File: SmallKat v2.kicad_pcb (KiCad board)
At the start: 2 copper layers, 90 x 56 mm, 64 parts, among them IC1 TPS562201DDCR, J1 Conn_01x06_Male, J10 Conn_01x03_Male, J11 Conn_01x03_Male, J12 Conn_01x03_Male, J13 Conn_01x03_Male, J14 Conn_01x03_Male, J15 Conn_01x03_Male, J16 Conn_01x03_Male, J17 Conn_01x03_Male, J18 Conn_01x03_Male, J19 Conn_01x03_Male, J2 Conn_01x06_Male, J20 Conn_01x03_Male, J21 Conn_01x02_Male, J22 Conn_01x02_Male, J23 Conn_01x02_Male, J24 Conn_01x02_Male, J25 Conn_01x02_Male, J26 Conn_01x02_Male, J27 Conn_01x02_Male, J28 Conn_01x02_Male, J29 Conn_01x02_Male, J3 Conn_01x06_Male, J30 Conn_01x15_Female, J31 Conn_01x15_Female, J4 Conn_01x06_Male, J5 Conn_01x03_Male, J6 Conn_01x03_Male, J7 Conn_01x03_Male, J8 Conn_01x03_Male, J9 Conn_01x03_Male, U3 PCA9685BS, U4 BNO055, Y1 32.768kHz

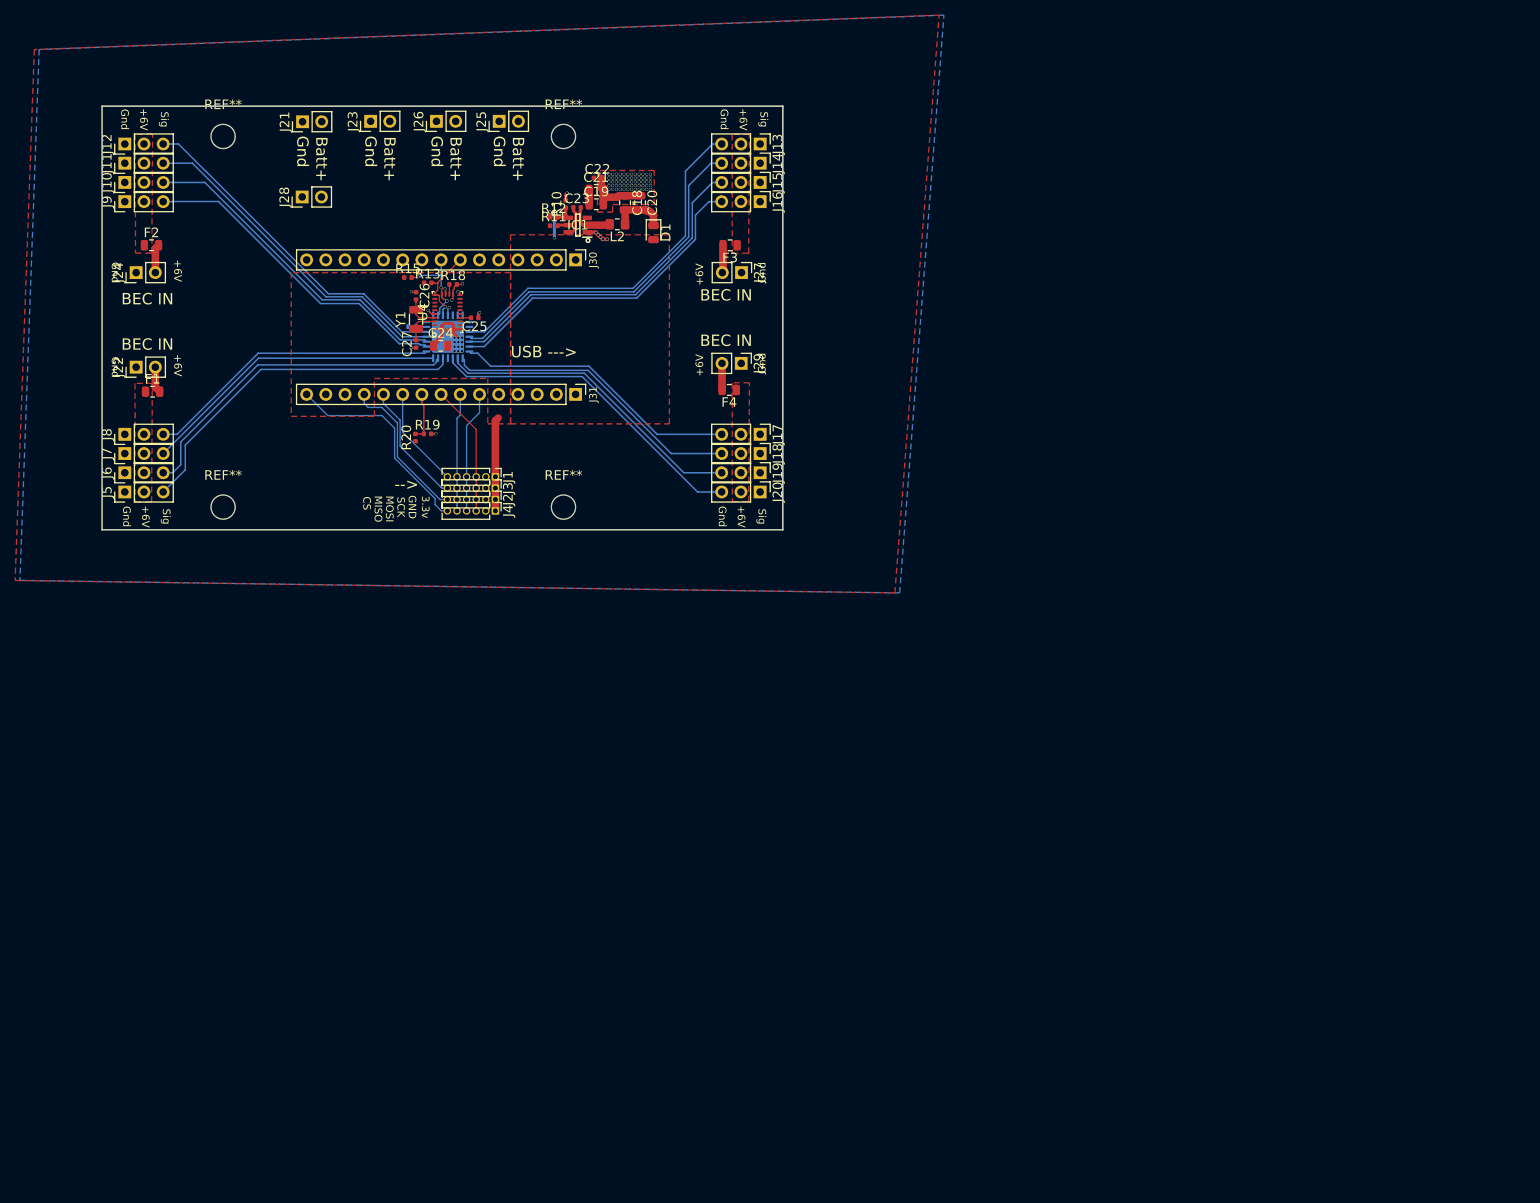
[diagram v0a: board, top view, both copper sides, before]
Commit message: init
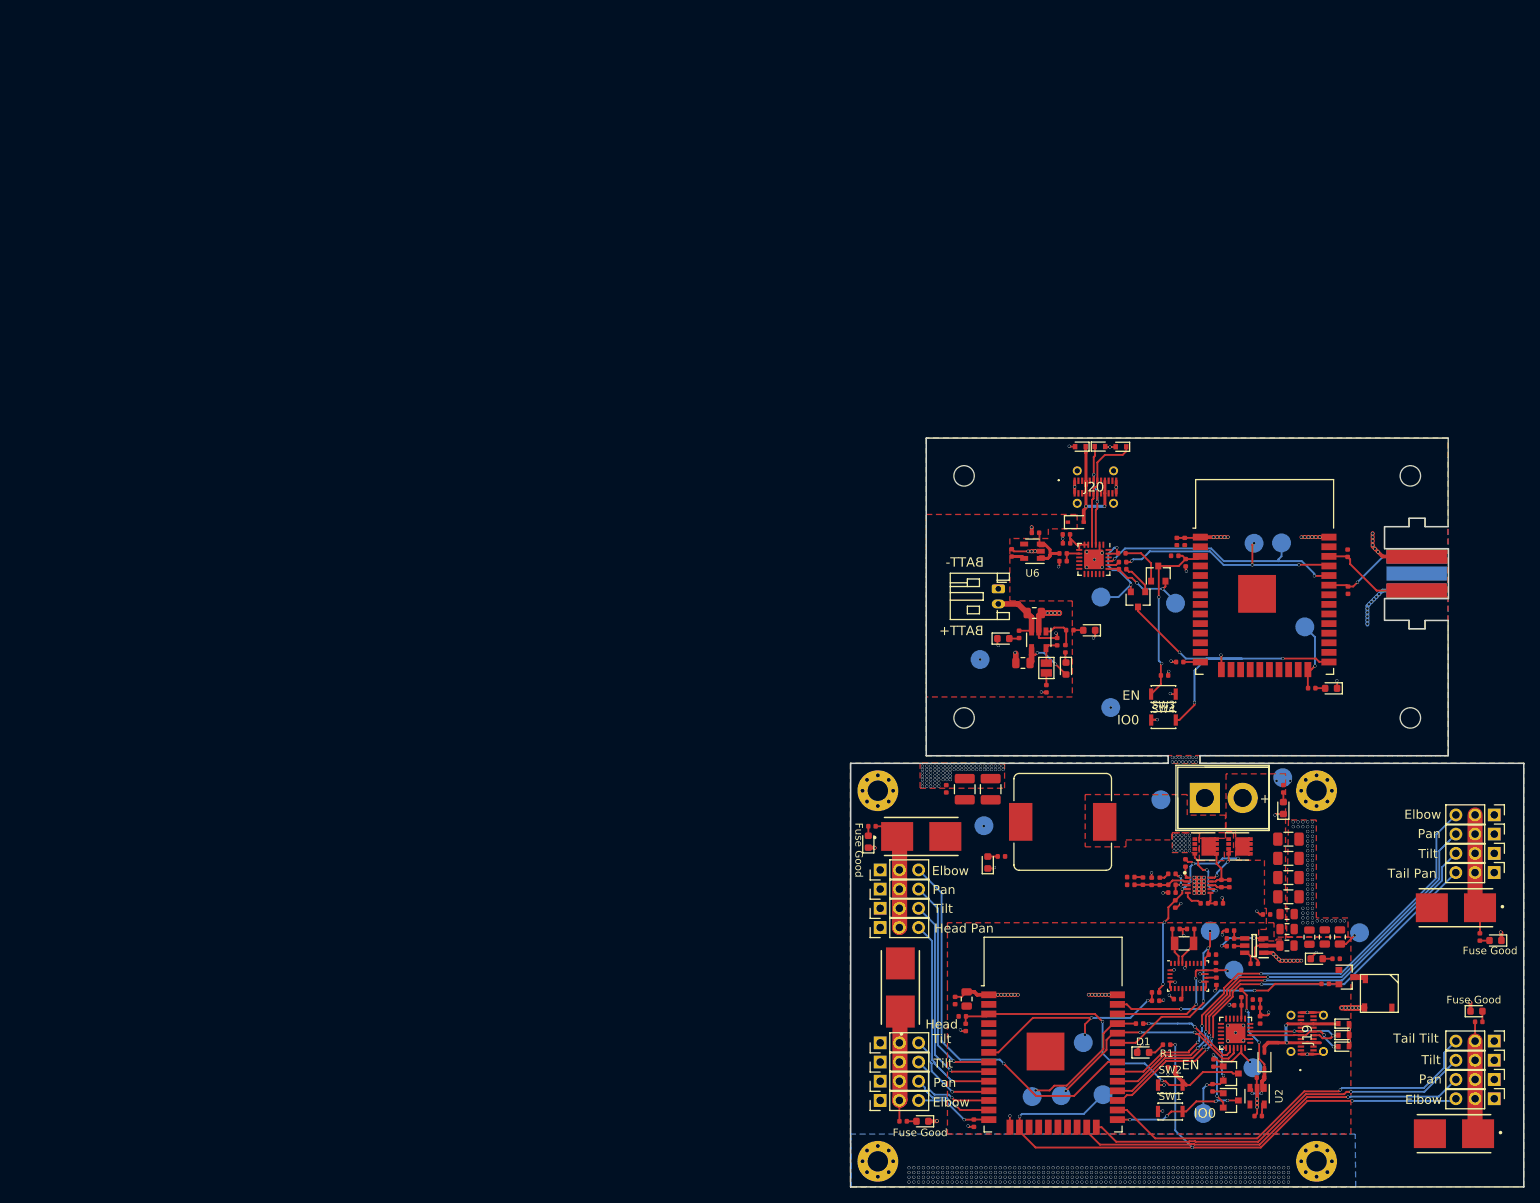
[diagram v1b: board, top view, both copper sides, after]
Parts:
- removed J21, J22, J23, J24, J25, J26, J27, J28, J29: Conn_01x02_Male, Connector_PinHeader_2.54mm:PinHeader_1x02_P2.54mm_Vertical
- removed J30, J31: Conn_01x15_Female, Connector_PinHeader_2.54mm:PinHeader_1x15_P2.54mm_Vertical
- removed REF** (x4): MountingHole_3.2mm_M3, MountingHole:MountingHole_3.2mm_M3
- added BZ1: Buzzer, KLJ-5030:KLJ-5030, F.Cu at (168.9, 117.3)
- added C1: 10uF, Capacitor_SMD:C_0805_2012Metric, F.Cu at (156.7, 108.8)
- added C10: 1000pF, Capacitor_SMD:C_0402_1005Metric, F.Cu at (136.0, 101.9)
- added C11: 100pF, Capacitor_SMD:C_0402_1005Metric, F.Cu at (141.4, 102.9)
- added C12: 10nF, Capacitor_SMD:C_0402_1005Metric, F.Cu at (141.4, 101.5)
- added C13: 1uF, Capacitor_SMD:C_0402_1005Metric, F.Cu at (141.9, 105.5)
- added C14: 4.7uF, Capacitor_SMD:C_0402_1005Metric, F.Cu at (147.7, 105.4)
- added C15: 470nF, Capacitor_SMD:C_0402_1005Metric, F.Cu at (148.0, 102.8)
- added C16: 10uF, Capacitor_SMD:C_1206_3216Metric, F.Cu at (156.8, 104.5)
- added C17: 47uF, Capacitor_SMD:C_1206_3216Metric, F.Cu at (156.8, 96.9)
- added C2: 10uF, Capacitor_SMD:C_0805_2012Metric, F.Cu at (156.7, 106.8)
- added C28: 0.1uF, Capacitor_SMD:C_0402_1005Metric, F.Cu at (152.6, 118.1)
- added C29: 0.1uF, Capacitor_SMD:C_0402_1005Metric, F.Cu at (153.1, 120.8)
- added C3: 22uF, Capacitor_SMD:C_0805_2012Metric, F.Cu at (161.6, 109.8)
- added C31: 0.1uF, Capacitor_SMD:C_0402_1005Metric, F.Cu at (141.4, 127.1)
- added C32: 0.1uF, Capacitor_SMD:C_0402_1005Metric, F.Cu at (114.2, 121.8)
- added C33: 10uF, Capacitor_SMD:C_0805_2012Metric, F.Cu at (121.7, 73.6)
- added C34: 10uF, Capacitor_SMD:C_0805_2012Metric, F.Cu at (123.2, 67.0)
- added C35: 1uF, Capacitor_SMD:C_0402_1005Metric, F.Cu at (123.4, 56.4)
- added C36: 22uF, Capacitor_SMD:C_0805_2012Metric, F.Cu at (163.7, 109.8)
- added C37: 1uF, Capacitor_SMD:C_0402_1005Metric, F.Cu at (120.2, 59.0)
- added C38: 0.1uF, Capacitor_SMD:C_0402_1005Metric, F.Cu at (143.1, 57.6)
- added C39: 4.7uF, Capacitor_SMD:C_0402_1005Metric, F.Cu at (142.1, 57.6)
- added C4: 0.1uF, Capacitor_SMD:C_0402_1005Metric, F.Cu at (153.9, 106.9)
- added C40: 0.1uF, Capacitor_SMD:C_0402_1005Metric, F.Cu at (127.5, 57.8)
- added C41: 0.1uF, Capacitor_SMD:C_0402_1005Metric, F.Cu at (127.5, 56.6)
- added C43: 0.1uF, Capacitor_SMD:C_0402_1005Metric, F.Cu at (140.5, 75.3)
- added C44: 0.1uF, Capacitor_SMD:C_0402_1005Metric, F.Cu at (143.3, 60.4)
- added C5: 22uF, Capacitor_SMD:C_0805_2012Metric, F.Cu at (159.6, 109.9)
- added C6: 0.1uF, Capacitor_SMD:C_0402_1005Metric, F.Cu at (152.3, 113.4)
- added C7: 0.1uF, Capacitor_SMD:C_0402_1005Metric, F.Cu at (142.2, 118.0)
- added C8: 10pF, Capacitor_SMD:C_0402_1005Metric, F.Cu at (143.9, 108.8)
- added C9: 10pF, Capacitor_SMD:C_0402_1005Metric, F.Cu at (142.0, 108.8)
- added D10: LED, LED_SMD:LED_0603_1608Metric, F.Cu at (119.2, 70.4)
- added D11: LED, LED_SMD:LED_0603_1608Metric, F.Cu at (127.4, 74.3)
- added D12: LED, LED_SMD:LED_0603_1608Metric, F.Cu at (130.5, 69.3)
- added D13: D_TVS, Diode_SMD:D_SOD-523, F.Cu at (129.3, 45.0)
- added D14: D_Schottky, Diode_SMD:D_SOD-323, F.Cu at (128.7, 55.0)
- added D15: D_TVS, Diode_SMD:D_SOD-523, F.Cu at (134.7, 45.0)
- added D16: D_TVS, Diode_SMD:D_SOD-523, F.Cu at (131.9, 45.0)
- added D17: LED, LED_SMD:LED_0603_1608Metric, F.Cu at (108.5, 134.2)
- added D18: LED, LED_SMD:LED_0603_1608Metric, F.Cu at (101.3, 97.2)
- added D19: LED, LED_SMD:LED_0603_1608Metric, F.Cu at (181.7, 119.7)
- added D2: LED, LED_SMD:LED_0603_1608Metric, F.Cu at (156.2, 92.8)
- added D20: LED, LED_SMD:LED_0603_1608Metric, F.Cu at (184.2, 110.3)
- added D3: LED, LED_SMD:LED_0603_1608Metric, F.Cu at (160.6, 112.7)
- added D4: LED, LED_SMD:LED_0603_1608Metric, F.Cu at (117.1, 100.0)
- added D5: D_TVS, Diode_SMD:D_SOD-523, F.Cu at (164.1, 121.3)
- added D6: D_Schottky, Diode_SMD:D_SOD-323, F.Cu at (153.7, 126.1)
- added D7: D_TVS, Diode_SMD:D_SOD-523, F.Cu at (164.1, 122.8)
- added D8: D_TVS, Diode_SMD:D_SOD-523, F.Cu at (164.1, 124.3)
- added D9: LED, LED_SMD:LED_0603_1608Metric, F.Cu at (162.5, 77.0)
- added H1: MountingHole_Pad, MountingHole:MountingHole_2.7mm_M2.5_Pad_Via, F.Cu at (160.6, 139.5)
- added H2: MountingHole_Pad, MountingHole:MountingHole_2.7mm_M2.5_Pad_Via, F.Cu at (102.6, 139.5)
- added H3: MountingHole_Pad, MountingHole:MountingHole_2.7mm_M2.5_Pad_Via, F.Cu at (160.6, 90.5)
- added H4: MountingHole_Pad, MountingHole:MountingHole_2.7mm_M2.5_Pad_Via, F.Cu at (102.6, 90.5)
- added H5: MountingHole, MountingHole:MountingHole_2.7mm_M2.5, F.Cu at (114.0, 48.9)
- added H6: MountingHole, MountingHole:MountingHole_2.7mm_M2.5, F.Cu at (173.0, 48.9)
- added H7: MountingHole, MountingHole:MountingHole_2.7mm_M2.5, F.Cu at (114.0, 80.9)
- added H8: MountingHole, MountingHole:MountingHole_2.7mm_M2.5, F.Cu at (173.0, 80.9)
- added IC2: TPS40192DRCT, TPS40192DRCT:SON50P300X300X100-11N, F.Cu at (145.0, 103.0)
- added JP1: Jumper_NO_Small, Jumper:SolderJumper-2_P1.3mm_Open_Pad1.0x1.5mm, F.Cu at (124.8, 74.3)
- added L1: 4.7uH, Inductor_SMD:L_0805_2012Metric, F.Cu at (156.6, 111.0)
- added Q1: BUK9M120-100EX, Package_SON:VSON-8_3.3x3.3mm_P0.65mm_NexFET, F.Cu at (150.4, 97.9)
- added Q2: BUK9M120-100EX, Package_SON:VSON-8_3.3x3.3mm_P0.65mm_NexFET, F.Cu at (145.9, 97.9)
- added Q3: MMBT3904, Package_TO_SOT_SMD:SOT-23, F.Cu at (149.2, 127.9)
- added Q4: MMBT3904, Package_TO_SOT_SMD:SOT-23, F.Cu at (149.2, 131.4)
- added Q5: MMBT3904, Package_TO_SOT_SMD:SOT-23, F.Cu at (139.6, 61.8)
- added Q6: MMBT3904, Package_TO_SOT_SMD:SOT-23, F.Cu at (137.0, 65.2)
- added Q7: 2N3905, Package_TO_SOT_SMD:SOT-23, F.Cu at (164.5, 115.1)
- added R1: R, Resistor_SMD:R_0402_1005Metric, F.Cu at (140.7, 124.1)
- added R16: 3.9k, Resistor_SMD:R_0402_1005Metric, F.Cu at (141.4, 104.0)
- added R17: 100k, Resistor_SMD:R_0402_1005Metric, F.Cu at (143.2, 100.1)
- added R2: 10K, Resistor_SMD:R_0402_1005Metric, F.Cu at (139.3, 118.3)
- added R21: 10K, Resistor_SMD:R_0402_1005Metric, F.Cu at (115.3, 134.5)
- added R22: 10K, Resistor_SMD:R_0402_1005Metric, F.Cu at (150.6, 117.3)
- added R23: 20K, Resistor_SMD:R_0402_1005Metric, F.Cu at (150.2, 118.9)
- added R24: 470R, Resistor_SMD:R_0402_1005Metric, F.Cu at (137.2, 121.3)
- added R25: 10K, Resistor_SMD:R_0402_1005Metric, F.Cu at (146.9, 126.5)
- added R26: 10K, Resistor_SMD:R_0402_1005Metric, F.Cu at (146.8, 129.8)
- added R27: 10K, Resistor_SMD:R_0402_1005Metric, F.Cu at (113.7, 120.3)
- added R28: 330R, Resistor_SMD:R_0402_1005Metric, F.Cu at (159.9, 76.9)
- added R29: 10K, Resistor_SMD:R_0402_1005Metric, F.Cu at (164.7, 59.1)
- added R3: 6.2k, Resistor_SMD:R_0402_1005Metric, F.Cu at (139.3, 117.2)
- added R30: 10K, Resistor_SMD:R_0402_1005Metric, F.Cu at (164.7, 64.0)
- added R31: 330R, Resistor_SMD:R_0402_1005Metric, F.Cu at (121.2, 69.8)
- added R32: 10K, Resistor_SMD:R_0402_1005Metric, F.Cu at (126.3, 70.8)
- added R33: 2.5K, Resistor_SMD:R_0402_1005Metric, F.Cu at (124.8, 77.0)
- added R34: 470R, Resistor_SMD:R_0402_1005Metric, F.Cu at (127.4, 71.7)
- added R35: 470R, Resistor_SMD:R_0402_1005Metric, F.Cu at (127.9, 69.3)
- added R36: 10K, Resistor_SMD:R_0402_1005Metric, F.Cu at (142.5, 73.5)
- added R37: 10K, Resistor_SMD:R_0402_1005Metric, F.Cu at (127.1, 59.1)
- added R38: 20K, Resistor_SMD:R_0402_1005Metric, F.Cu at (127.0, 60.1)
- added R39: 470R, Resistor_SMD:R_0402_1005Metric, F.Cu at (134.9, 60.3)
- added R4: 10K, Resistor_SMD:R_0402_1005Metric, F.Cu at (147.3, 113.7)
- added R40: 10K, Resistor_SMD:R_0402_1005Metric, F.Cu at (134.8, 59.1)
- added R41: 10K, Resistor_SMD:R_0402_1005Metric, F.Cu at (134.9, 61.2)
- added R42: 10K, Resistor_SMD:R_0402_1005Metric, F.Cu at (141.8, 59.4)
- added R43: 10K, Resistor_SMD:R_0402_1005Metric, F.Cu at (161.7, 116.0)
- added R44: R, Resistor_SMD:R_0402_1005Metric, F.Cu at (105.9, 134.2)
- added R45: R, Resistor_SMD:R_0402_1005Metric, F.Cu at (101.8, 95.2)
- added R46: R, Resistor_SMD:R_0402_1005Metric, F.Cu at (182.0, 121.0)
- added R47: R, Resistor_SMD:R_0402_1005Metric, F.Cu at (182.2, 109.8)
- added R5: 10K, Resistor_SMD:R_0402_1005Metric, F.Cu at (146.8, 112.2)
- added R6: 4.7K, Resistor_SMD:R_0402_1005Metric, F.Cu at (156.2, 90.2)
- added R7: 330R, Resistor_SMD:R_0402_1005Metric, F.Cu at (163.1, 112.7)
- added R8: 10K, Resistor_SMD:R_0402_1005Metric, F.Cu at (149.2, 109.0)
- added R9: 33.2K, Resistor_SMD:R_0402_1005Metric, F.Cu at (149.2, 110.0)
- added SW1: SW_SPST, Button_Switch_SMD:SW_SPST_CK_KXT3, F.Cu at (141.2, 132.9)
- added SW2: SW_SPST, Button_Switch_SMD:SW_SPST_CK_KXT3, F.Cu at (141.2, 129.4)
- added SW3: SW_SPST, Button_Switch_SMD:SW_SPST_CK_KXT3, F.Cu at (140.3, 81.2)
- added SW4: SW_SPST, Button_Switch_SMD:SW_SPST_CK_KXT3, F.Cu at (140.3, 77.7)
- added TP1: TestPoint, TestPoint:TestPoint_Pad_D2.5mm, B.Cu at (132.3, 130.7)
- added TP10: TestPoint, TestPoint:TestPoint_Pad_D2.5mm, B.Cu at (126.8, 130.8)
- added TP11: TestPoint, TestPoint:TestPoint_Pad_D2.5mm, B.Cu at (152.1, 127.1)
- added TP12: TestPoint, TestPoint:TestPoint_Pad_D2.5mm, B.Cu at (145.6, 133.2)
- added TP13: TestPoint, TestPoint:TestPoint_Pad_D2.5mm, B.Cu at (152.3, 57.8)
- added TP14: TestPoint, TestPoint:TestPoint_Pad_D2.5mm, B.Cu at (155.9, 57.7)
- added TP15: TestPoint, TestPoint:TestPoint_Pad_D2.5mm, B.Cu at (132.1, 64.9)
- added TP16: TestPoint, TestPoint:TestPoint_Pad_D2.5mm, B.Cu at (141.9, 65.7)
- added TP17: TestPoint, TestPoint:TestPoint_Pad_D2.5mm, B.Cu at (116.1, 73.2)
- added TP18: TestPoint, TestPoint:TestPoint_Pad_D2.5mm, B.Cu at (133.3, 79.5)
- added TP19: TestPoint, TestPoint:TestPoint_Pad_D2.5mm, B.Cu at (159.0, 68.8)
- added TP2: TestPoint, TestPoint:TestPoint_Pad_D2.5mm, B.Cu at (146.5, 109.0)
- added TP3: TestPoint, TestPoint:TestPoint_Pad_D2.5mm, B.Cu at (149.6, 114.2)
- added TP4: TestPoint, TestPoint:TestPoint_Pad_D2.5mm, B.Cu at (129.7, 123.8)
- added TP5: TestPoint, TestPoint:TestPoint_Pad_D2.5mm, B.Cu at (166.2, 109.3)
- added TP6: TestPoint, TestPoint:TestPoint_Pad_D2.5mm, B.Cu at (156.1, 88.8)
- added TP7: TestPoint, TestPoint:TestPoint_Pad_D2.5mm, B.Cu at (140.0, 91.7)
- added TP8: TestPoint, TestPoint:TestPoint_Pad_D2.5mm, B.Cu at (116.6, 95.1)
- added TP9: TestPoint, TestPoint:TestPoint_Pad_D2.5mm, B.Cu at (123.0, 130.9)
- added U1: BNO055, Package_LGA:LGA-28_5.2x3.8mm_P0.5mm, F.Cu at (143.6, 115.0)
- added U2: MIC5365-3.3YC5, Package_TO_SOT_SMD:SOT-23-5, F.Cu at (152.7, 130.9)
- added U5: MCP73831-2-OT, Package_TO_SOT_SMD:SOT-23-5, F.Cu at (123.8, 70.5)
- added U6: MIC5365-3.3YC5, Package_TO_SOT_SMD:SOT-23-5, F.Cu at (123.0, 58.8)
- added U7: ESP32-WROOM-32, RF_Module:ESP32-WROOM-32, F.Cu at (153.7, 65.2)
- added U8: CP2102N-A01-GQFN24, Package_DFN_QFN:QFN-24-1EP_4x4mm_P0.5mm_EP2.6x2.6mm, F.Cu at (131.1, 59.9)
- added U9: WIICHUCK, WIICHUCK:CHUCK, F.Cu at (169.5, 61.8)
- C18: value 22uF -> 10uF; footprint Capacitor_SMD:C_0805_2012Metric -> Capacitor_SMD:C_1206_3216Metric
- C19: value 10Uf -> 100uF; footprint Capacitor_SMD:C_0805_2012Metric -> Capacitor_SMD:C_1210_3225Metric
- C20: value 22uF -> 47uF; footprint Capacitor_SMD:C_0805_2012Metric -> Capacitor_SMD:C_1206_3216Metric
- C21: value 10uF -> 100uF; footprint Capacitor_SMD:C_0805_2012Metric -> Capacitor_SMD:C_1210_3225Metric
- C22, C23, C25: value 0.1uF -> 1uF
- C24: value 10uF -> 22uF
- C26: value 10pF -> 0.1uF
- C27: value 10pF -> 4.7uF
- D1: value DIODE -> LED; footprint Diode_SMD:D_0805_2012Metric -> LED_SMD:LED_0603_1608Metric
- F1, F2, F3, F4: footprint Fuse:Fuse_0805_2012Metric -> 01550900M:0154.250DR
- J1, J2, J3, J4: value Conn_01x06_Male -> Conn_01x03_Male; footprint Connector_PinHeader_1.27mm:PinHeader_1x06_P1.27mm_Vertical -> Connector_PinHeader_2.54mm:PinHeader_1x03_P2.54mm_Vertical
- J18: value Conn_01x03_Male -> Conn_01x02_Male; footprint Connector_PinHeader_2.54mm:PinHeader_1x03_P2.54mm_Vertical -> Connector_JST:JST_PH_S2B-PH-K_1x02_P2.00mm_Horizontal
- J19, J20: value Conn_01x03_Male -> USB_C_Receptacle; footprint Connector_PinHeader_2.54mm:PinHeader_1x03_P2.54mm_Vertical -> U263-241N-4BQC11-1:U263241N4BQC111
- J9: value Conn_01x03_Male -> Conn_01x02_Male; footprint Connector_PinHeader_2.54mm:PinHeader_1x03_P2.54mm_Vertical -> SmallKat ESP32:SHDR2W320P716_1X2_1574X813X1588P
- L2: value 4.7uH -> 1uH; footprint Inductor_SMD:L_0805_2012Metric_Pad1.15x1.40mm_HandSolder -> Inductor_SMD:L_Bourns_SRP1245A
- R12: value 61.63k -> 2.18k
- R13: value 10K -> 20k
- R14: value 10K -> 2.61k; moved to F.Cu
- R15: value 10K -> 4.22k
- R18, R19: value 10K -> 100k
- R20: value 6.2k -> 1K
- U3: value PCA9685BS -> ESP32-WROOM-32; footprint Package_DFN_QFN:QFN-28-1EP_6x6mm_P0.65mm_EP4.25x4.25mm -> RF_Module:ESP32-WROOM-32; moved to F.Cu
- U4: value BNO055 -> CP2102N-A01-GQFN24; footprint Package_LGA:LGA-28_5.2x3.8mm_P0.5mm -> Package_DFN_QFN:QFN-24-1EP_4x4mm_P0.5mm_EP2.6x2.6mm
- moved J10 217.8 mm to (184.1, 131.2), turned to 270 degrees
- moved J11 217.8 mm to (184.1, 128.7), turned to 270 degrees
- moved J12 217.8 mm to (184.1, 126.1), turned to 270 degrees
- moved J9 163.1 mm to (145.8, 91.5), turned to 0 degrees
- moved J13 153.2 mm to (184.1, 123.6)
- moved F3 151.5 mm to (178.7, 135.8)
- moved C25 147.9 mm to (152.8, 133.5)
- moved C23 146.3 mm to (153.1, 128.4), turned to 180 degrees
- moved C27 141.6 mm to (152.6, 119.2), turned to 0 degrees
- moved U4 141.2 mm to (149.9, 122.6), turned to 180 degrees
- moved J14 135.0 mm to (184.0, 101.3)
- moved R11 132.9 mm to (147.3, 115.7), turned to 270 degrees
- moved R10 131.7 mm to (149.2, 111.0), turned to 0 degrees
- moved J15 131.5 mm to (184.1, 98.8)
- moved Y1 130.8 mm to (143.0, 110.7), turned to 0 degrees
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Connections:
- C18 pad 1: GND -> +BATT
- C18 pad 2: Net-(C18-Pad2) -> GND
- C19 pad 1: +BATT -> +6V
- C20 pad 1: GND -> +BATT
- C20 pad 2: Net-(C18-Pad2) -> GND
- C21 pad 1: +BATT -> +6V
- C22 pad 1: +BATT -> +6V
- C23 pad 1: Net-(C23-Pad1) -> +5V
- C23 pad 2: Net-(C23-Pad2) -> GND
- C24 pad 1: GND -> +3V3
- C24 pad 2: +3V3 -> GND
- C25 pad 1: GND -> +3V3
- C25 pad 2: Net-(C25-Pad2) -> GND
- C26 pad 1: GND -> +3V3
- C26 pad 2: Net-(C26-Pad2) -> GND
- C27 pad 1: GND -> +3V3
- C27 pad 2: Net-(C27-Pad2) -> GND
- D1 pad 1: Net-(C18-Pad2) -> GND
- D1 pad 2: +5V -> Net-(D1-Pad2)
- F1 pad 1: +6V_1 -> Net-(F1-Pad1)
- F1 pad 2: +6V_IN1 -> +6V
- F2 pad 1: +6V_2 -> Net-(F2-Pad1)
- F2 pad 2: +6V_IN2 -> +6V
- F3 pad 1: +6V_3 -> Net-(F3-Pad1)
- F3 pad 2: +6V_IN3 -> +6V
- F4 pad 1: +6V_4 -> Net-(F4-Pad1)
- F4 pad 2: +6V_IN4 -> +6V
- IC1 pad 2: Net-(C23-Pad2) -> Net-(C6-Pad2)
- IC1 pad 6: Net-(C23-Pad1) -> Net-(C6-Pad1)
- J1 pad 1: +3V3 -> GND
- J1 pad 2: GND -> Net-(F1-Pad1)
- J1 pad 3: SCK -> /MainBoard/SERVO0
- J10 pad 2: +6V_2 -> Net-(F3-Pad1)
- J10 pad 3: SERVO5 -> /MainBoard/SERVO8
- J11 pad 2: +6V_2 -> Net-(F3-Pad1)
- J11 pad 3: SERVO6 -> /MainBoard/SERVO9
- J12 pad 2: +6V_2 -> Net-(F3-Pad1)
- J12 pad 3: SERVO7 -> /MainBoard/SERVO10
- J13 pad 2: +6V_3 -> Net-(F3-Pad1)
- J13 pad 3: SERVO8 -> /MainBoard/SERVO11
- J14 pad 2: +6V_3 -> Net-(F4-Pad1)
- J14 pad 3: SERVO9 -> /MainBoard/SERVO12
- J15 pad 2: +6V_3 -> Net-(F4-Pad1)
- J15 pad 3: SERVO10 -> /MainBoard/SERVO13
- J16 pad 2: +6V_3 -> Net-(F4-Pad1)
- J16 pad 3: SERVO11 -> /MainBoard/SERVO14
- J17 pad 2: +6V_4 -> Net-(F4-Pad1)
- J17 pad 3: SERVO12 -> /MainBoard/SERVO15
- J18 pad 2: +6V_4 -> +3V8
- J2 pad 1: +3V3 -> GND
- J2 pad 2: GND -> Net-(F1-Pad1)
- J2 pad 3: SCK -> /MainBoard/SERVO1
- J3 pad 1: +3V3 -> GND
- J3 pad 2: GND -> Net-(F1-Pad1)
- J3 pad 3: SCK -> /MainBoard/SERVO2
- J4 pad 1: +3V3 -> GND
- J4 pad 2: GND -> Net-(F1-Pad1)
- J4 pad 3: SCK -> /MainBoard/SERVO3
- J5 pad 2: +6V_1 -> Net-(F2-Pad1)
- J5 pad 3: SERVO0 -> /MainBoard/SERVO4
- J6 pad 2: +6V_1 -> Net-(F2-Pad1)
- J6 pad 3: SERVO1 -> /MainBoard/SERVO5
- J7 pad 2: +6V_1 -> Net-(F2-Pad1)
- J7 pad 3: SERVO2 -> /MainBoard/SERVO6
- J8 pad 2: +6V_1 -> Net-(F2-Pad1)
- J8 pad 3: SERVO3 -> /MainBoard/SERVO7
- J9 pad 2: +6V_2 -> +BATT
- L2 pad 1: Net-(C18-Pad2) -> Net-(C15-Pad1)
- L2 pad 2: Net-(C23-Pad2) -> +6V
- R10 pad 1: Net-(IC1-Pad4) -> +BATT
- R10 pad 2: GND -> Net-(IC1-Pad5)
- R11 pad 1: +BATT -> Net-(R11-Pad1)
- R11 pad 2: Net-(IC1-Pad5) -> GND
- R12 pad 1: +5V -> Net-(C11-Pad2)
- R12 pad 2: Net-(IC1-Pad4) -> GND
- R13 pad 1: +3V3 -> +6V
- R13 pad 2: SDA -> Net-(C11-Pad2)
- R14 pad 1: Net-(R14-Pad1) -> Net-(C11-Pad2)
- R14 pad 2: GND -> Net-(C10-Pad2)
- R15 pad 1: +3V3 -> Net-(C12-Pad2)
- R15 pad 2: SCL -> Net-(C11-Pad2)
- R18 pad 1: Net-(R18-Pad1) -> Net-(C14-Pad1)
- R18 pad 2: GND -> Net-(IC2-Pad5)
- R19 pad 1: BATTMONITOR -> Net-(C15-Pad1)
- R19 pad 2: GND -> Net-(C15-Pad2)
- R20 pad 1: +BATT -> +6V
- R20 pad 2: BATTMONITOR -> Net-(D4-Pad2)
- U3 pad 1: (no net) -> GND
- U3 pad 10: SERVO15 -> /MainBoard/SERVO4
- U3 pad 11: GND -> /MainBoard/SERVO3
- U3 pad 12: SERVO0 -> /MainBoard/SERVO2
- U3 pad 13: SERVO1 -> /MainBoard/SERVO1
- U3 pad 14: SERVO2 -> /MainBoard/SERVO0
- U3 pad 15: SERVO3 -> GND
- U3 pad 16: SERVO4 -> /MainBoard/SERVO8
- U3 pad 17: SERVO5 -> (no net)
- U3 pad 18: SERVO6 -> (no net)
- U3 pad 19: SERVO7 -> (no net)
- U3 pad 2: (no net) -> +3V3
- U3 pad 20: Net-(R14-Pad1) -> (no net)
- U3 pad 22: GND -> (no net)
- U3 pad 23: SCL -> /MainBoard/SERVO9
- U3 pad 24: SDA -> /MainBoard/SERVO10
- U3 pad 25: +3V3 -> /MainBoard/ESP32Module/IO0
- U3 pad 26: (no net) -> /MainBoard/SERVO11
- U3 pad 27: (no net) -> /MainBoard/SERVO12
- U3 pad 28: (no net) -> /MainBoard/SERVO13
- U3 pad 29: GND -> /MainBoard/SERVO14
- U3 pad 3: SERVO8 -> /MainBoard/ESP32Module/EN
- U3 pad 4: SERVO9 -> (no net)
- U3 pad 5: SERVO10 -> (no net)
- U3 pad 6: SERVO11 -> (no net)
- U3 pad 7: SERVO12 -> /MainBoard/BATTMONITOR
- U3 pad 8: SERVO13 -> /MainBoard/SERVO6
- U3 pad 9: SERVO14 -> /MainBoard/SERVO5
- U4 pad 15: GND -> (no net)
- U4 pad 16: GND -> (no net)
- U4 pad 17: Net-(R18-Pad1) -> (no net)
- U4 pad 18: GND -> (no net)
- U4 pad 19: SCL -> /MainBoard/ESP32Module/RTS
- U4 pad 20: SDA -> Net-(R24-Pad2)
- U4 pad 21: (no net) -> /MainBoard/ESP32Module/RXD
- U4 pad 23: (no net) -> /MainBoard/ESP32Module/DTR
- U4 pad 3: +3V3 -> /MainBoard/ESP32Module/USBD_P
- U4 pad 4: +3V3 -> /MainBoard/ESP32Module/USBD_N
- U4 pad 5: GND -> +3V3
- U4 pad 6: GND -> +3V3
- U4 pad 7: (no net) -> +3V3
- U4 pad 8: (no net) -> Net-(R22-Pad1)
- U4 pad 9: Net-(C25-Pad2) -> (no net)
- Y1 pad 1: Net-(C26-Pad2) -> Net-(C8-Pad2)
- Y1 pad 2: Net-(C27-Pad2) -> Net-(C9-Pad2)
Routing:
- net GND: track 28.5 -> 125.7 mm, vias 87 -> 315
- net /MainBoard/SERVO8: track 0.00 -> 90.6 mm, vias 0 -> 4
- net /MainBoard/SERVO15: track 0.00 -> 64.5 mm, vias 0 -> 3
- net /MainBoard/SERVO14: track 0.00 -> 62.8 mm, vias 0 -> 3
- net /MainBoard/SERVO13: track 0.00 -> 61.1 mm, vias 0 -> 3
- net /MainBoard/SERVO12: track 0.00 -> 59.7 mm, vias 0 -> 3
- net /MainBoard/SERVO9: track 0.00 -> 53.7 mm, vias 0 -> 1
- net /MainBoard/SERVO10: track 0.00 -> 52.8 mm, vias 0 -> 1
- net /MainBoard/SERVO11: track 0.00 -> 52.8 mm, vias 0 -> 1
- net /MainBoard/SERVO7: track 0.00 -> 52.0 mm, vias 0 -> 1
- net SERVO8: track 48.7 -> 0.00 mm
- net /MainBoard/ESP32Module/EN: track 0.00 -> 47.2 mm, vias 0 -> 2
- net SERVO9: track 47.0 -> 0.00 mm
- net SERVO0: track 46.7 -> 0.00 mm
- net SERVO7: track 45.1 -> 0.00 mm
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- added copper zone on B.Cu, net +6V
- added copper zone on F.Cu, net +6V
- added copper zone on F.Cu, net Net-(C15-Pad1)
- removed copper zone on F.Cu, net +6V_1
- removed copper zone on F.Cu, net +6V_2
- removed copper zone on F.Cu, net +6V_3
- removed copper zone on F.Cu, net +6V_4
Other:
- board size 90 x 56 mm -> 89 x 99 mm
- board text added: "+"
- board text added: "-"
- board text added: "5v"
- board text added: "6v"
- board text added: "BATT IN"
- board text added: "BATT+"
- board text added: "BATT-"
- board text added: "DTR"
- board text added: "EN"
- board text added: "Elbow"
- board text added: "Fuse Good"
- board text added: "Head Pan"
- board text added: "Head Tilt"
- board text added: "IO0"
- board text added: "IO19"
- board text added: "IO2"
- board text added: "Keion Bisland"
- board text added: "Pan"
- board text added: "RTS"
- board text added: "RX"
- board text added: "Rev 1.0"
- board text added: "SCL"
- board text added: "SDA"
- board text added: "SmallKat Mother Board"
- board text added: "SmallKat Remote Controller Board"
- board text added: "TX"
- board text added: "Tail Pan"
- board text added: "Tail Tilt"
- board text added: "Tilt"
- board text removed: "+6V"
- board text removed: "-->"
- board text removed: "BEC IN"
- board text removed: "Batt+"
- board text removed: "CS"
- board text removed: "Gnd"
- board text removed: "MISO"
- board text removed: "MOSI"
- board text removed: "Note to Kevin: If you plug something in backwards things will go poof. I have labeled everything as best I can but I cant prevent you from plugging in things backwards so its up to you now -Keion"
- board text removed: "SCK"
- board text removed: "Sig"
- board text removed: "SmallKat V2 Motherboard Rev 2. Keion Bisland Feb. 2019"
- board text removed: "USB --->"
